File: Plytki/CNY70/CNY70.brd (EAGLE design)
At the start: 23.8 x 24.1 mm, 5 parts

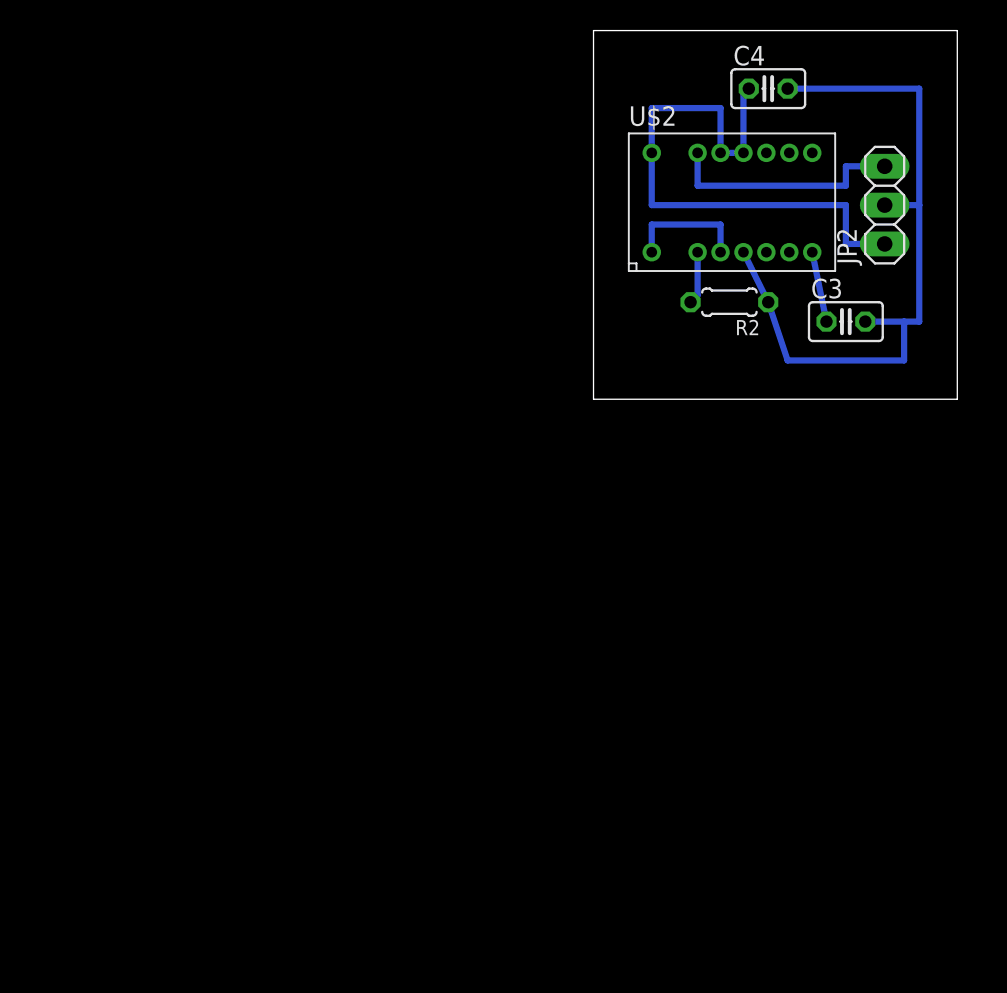
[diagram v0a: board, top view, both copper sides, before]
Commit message: Ostateczne projekty plytek
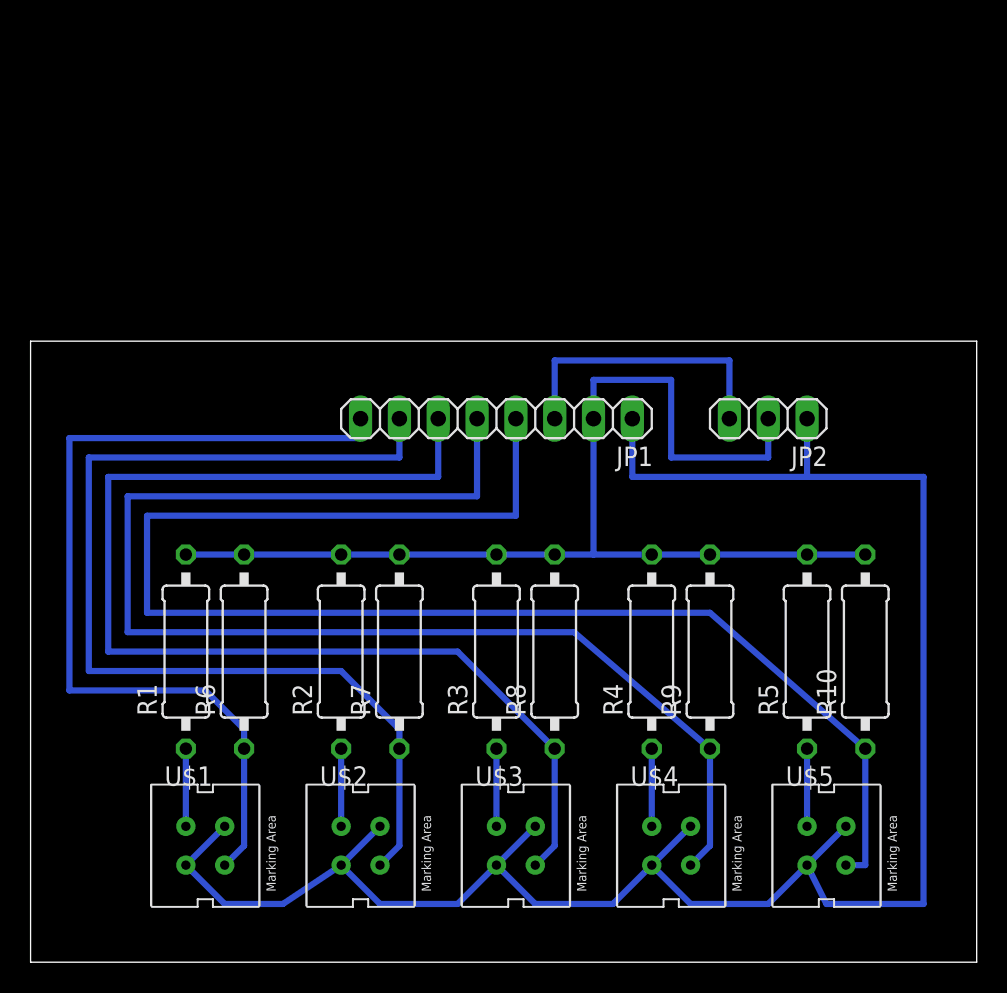
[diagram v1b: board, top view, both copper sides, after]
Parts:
- removed C3, C4: 0.1 μF, rcl:C025-025X050
- added JP1: (no value), pinhead:1X08
- added R1, R3, R4, R5: 100, rcl:0309/12
- added R10, R7, R8, R9: 10k, rcl:0309/12
- added R6: 10K, rcl:0309/12
- added U$1, U$3, U$4, U$5: CNY70, cny70:4
- R2: value (none) -> 100; device rcl:0204/5 -> rcl:0309/12
- U$2: value (none) -> CNY70; device SharpGP2Y0D810Z0F:LP16PIN -> cny70:4
- moved U$2 42.6 mm to (21.6, 7.62)
- moved R2 34.2 mm to (20.3, 20.3), turned to 90 degrees
- moved JP2 15.9 mm to (48.3, 35.6), turned to 180 degrees
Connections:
- removed net VCC: C4.1, JP2.1, U$2.11, U$2.12, U$2.14
- new net +5V: JP1.2, JP2.2, R1.2, R10.2, R2.2, R3.2, R4.2, R5.2, R6.2, R7.2, R8.2, R9.2
- new net N$1: R1.1, U$1.A
- new net N$10: JP1.4, R10.1, U$5.C
- new net N$12: JP1.5, R9.1, U$4.C
- new net N$2: R2.1, U$2.A
- new net N$3: R3.1, U$3.A
- new net N$4: R4.1, U$4.A
- new net N$9: JP1.3, JP2.3
- net GND: now also JP1.1, JP2.1, U$1.E, U$1.K, U$2.E, U$2.K, U$3.E, U$3.K, U$4.E, U$4.K, U$5.E, U$5.K; no longer C3.2, C4.2, JP2.2, R2.1, U$2.4
- net N$5: now also R5.1, U$5.A; no longer R2.2, U$2.2
- net N$6: now also JP1.8, R6.1, U$1.C; no longer C3.1, U$2.7
- net N$7: now also JP1.7, R7.1, U$2.C; no longer U$2.1, U$2.3
- net N$8: now also JP1.6, R8.1, U$3.C; no longer JP2.3, U$2.13
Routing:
- net N$10: track 0.00 -> 96.1 mm
- net N$12: track 0.00 -> 85.9 mm
- net GND: track 47.5 -> 130.5 mm
- net +5V: track 0.00 -> 74.9 mm
- net N$8: track 15.7 -> 76.8 mm
- net N$7: track 8.12 -> 68.1 mm
- net N$6: track 4.63 -> 58.7 mm
- net VCC: track 37.6 -> 0.00 mm
- net N$9: track 0.00 -> 19.0 mm
- net N$4: track 0.00 -> 5.08 mm
- net N$3: track 0.00 -> 5.08 mm
- net N$2: track 0.00 -> 5.08 mm
- net N$1: track 0.00 -> 5.08 mm
- net N$5: track 3.46 -> 5.08 mm
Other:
- board size 23.8 x 24.1 mm -> 61.9 x 40.6 mm
